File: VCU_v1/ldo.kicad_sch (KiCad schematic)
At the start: 8 parts, among them U3 AMS1117-3.3, U4 MIC5200-4.8YS

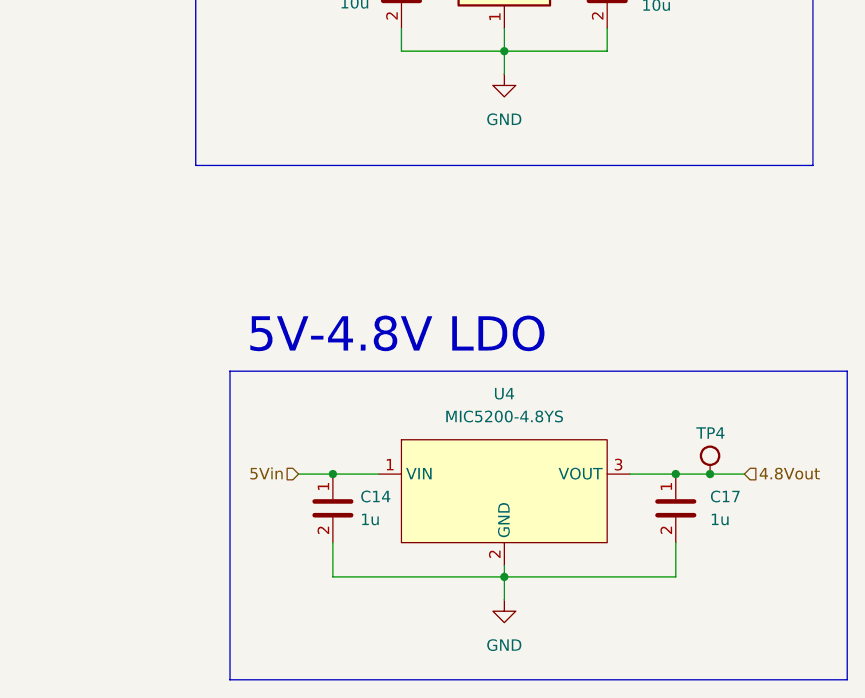
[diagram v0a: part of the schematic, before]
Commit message: omids wisdom came all over my power converters
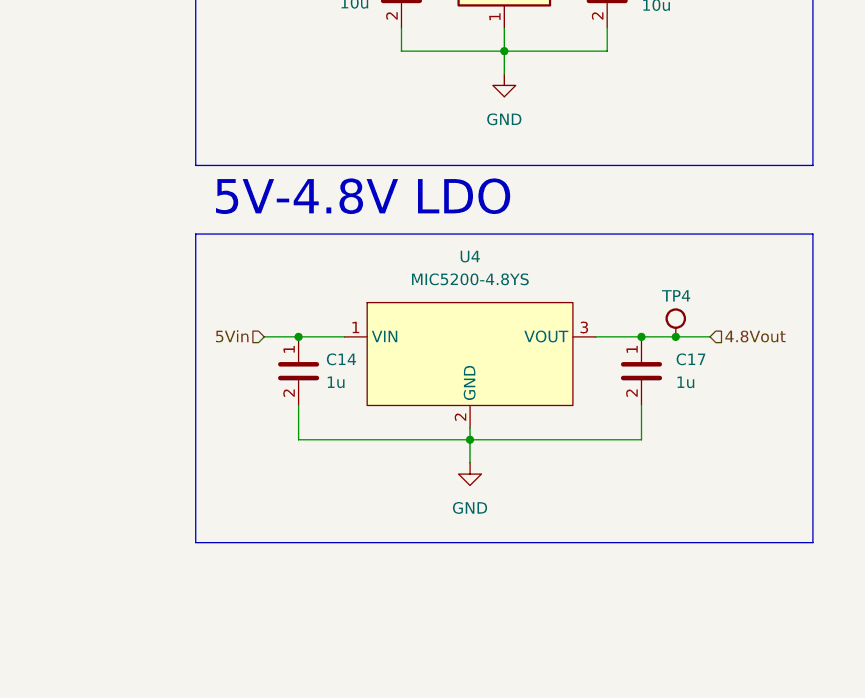
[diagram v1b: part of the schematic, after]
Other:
- moved on the sheet: C14, C17, TP4, U4
